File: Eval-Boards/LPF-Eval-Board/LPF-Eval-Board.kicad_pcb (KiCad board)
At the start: 2 copper layers, 38.1 x 20.3 mm, 3 parts

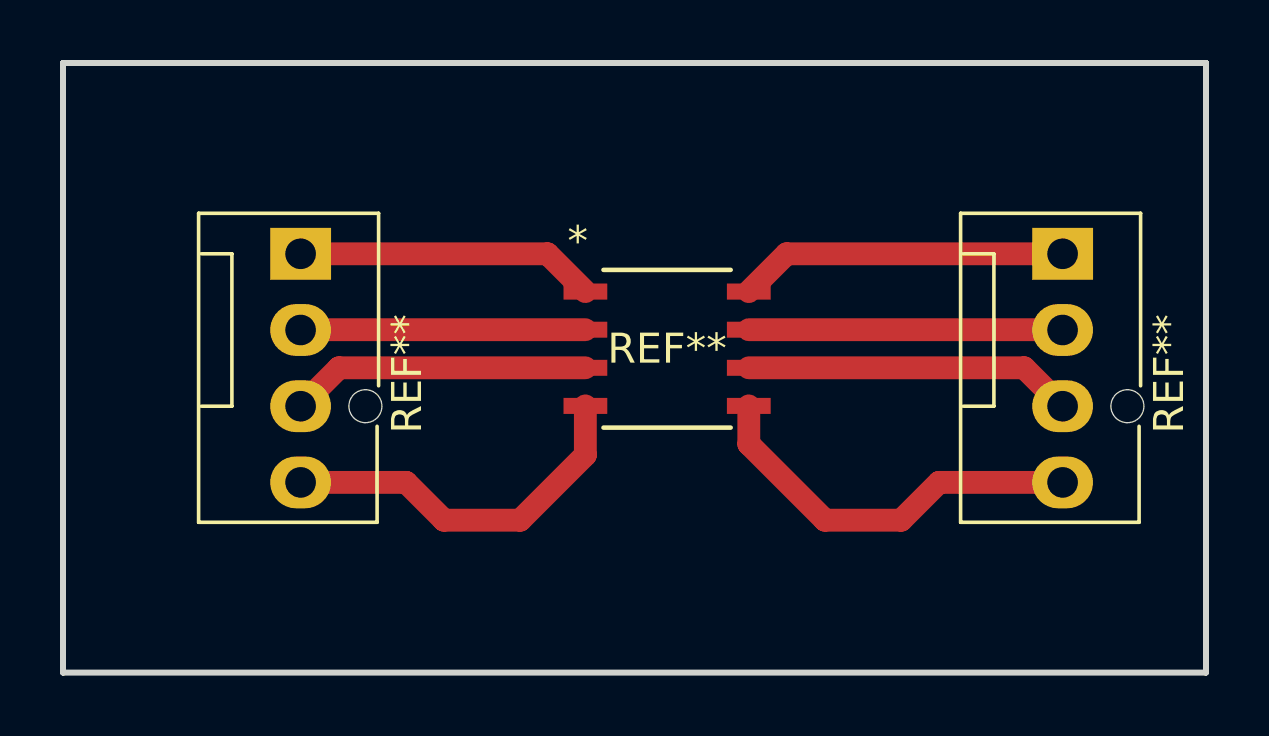
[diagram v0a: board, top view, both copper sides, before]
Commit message: :(
Finished eval boards
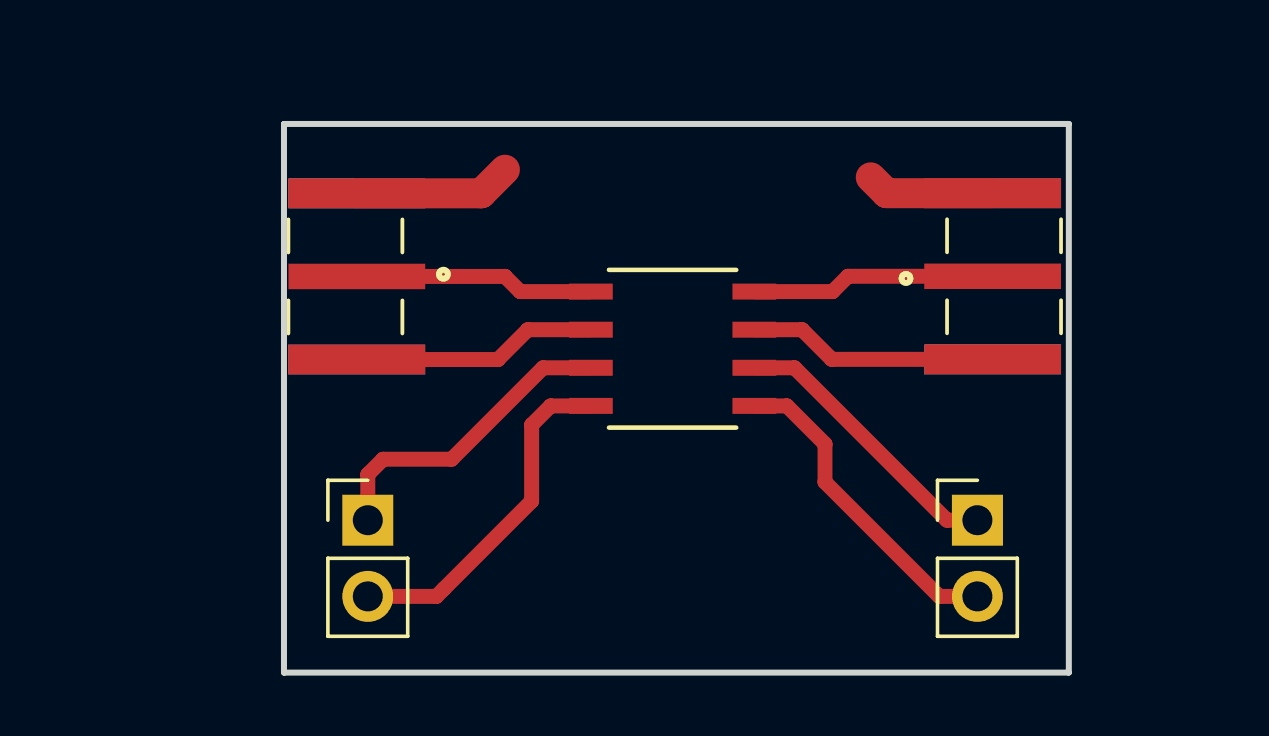
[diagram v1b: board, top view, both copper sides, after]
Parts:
- removed the REF** at (137.5, 77.5)
- removed the REF** at (162.9, 77.5)
- added REF**: TAOGLAS_EMPCB.SMAFSTJ.B.HT, SMA connectors:TAOGLAS_EMPCB.SMAFSTJ.B.HT, F.Cu at (139.3, 78.2)
- added REF**: PinHeader_1x02_P2.54mm_Vertical, Connector_PinHeader_2.54mm:PinHeader_1x02_P2.54mm_Vertical, F.Cu at (139.7, 86.4)
- added REF**: PinHeader_1x02_P2.54mm_Vertical, Connector_PinHeader_2.54mm:PinHeader_1x02_P2.54mm_Vertical, F.Cu at (160.0, 86.4)
- added REF**: TAOGLAS_EMPCB.SMAFSTJ.B.HT, SMA connectors:TAOGLAS_EMPCB.SMAFSTJ.B.HT, F.Cu at (160.5, 78.2)
- moved REF** 0.18 mm to (149.9, 80.6)
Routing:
- net (no net): track 88.4 -> 84.6 mm
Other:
- board size 38.1 x 20.3 mm -> 26.2 x 18.3 mm
